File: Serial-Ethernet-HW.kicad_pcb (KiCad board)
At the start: 4 copper layers, 41.1 x 50.7 mm, 52 parts, among them J1 7499111121A, J2 UJ2-MBH-1-SMT-TR, J3 D09P33E4GX00LF, U1 W5500, U2 MPM3612-33, U3 STM32G061GxUx, Y1 ECS-250-10-37B-CTN-TR

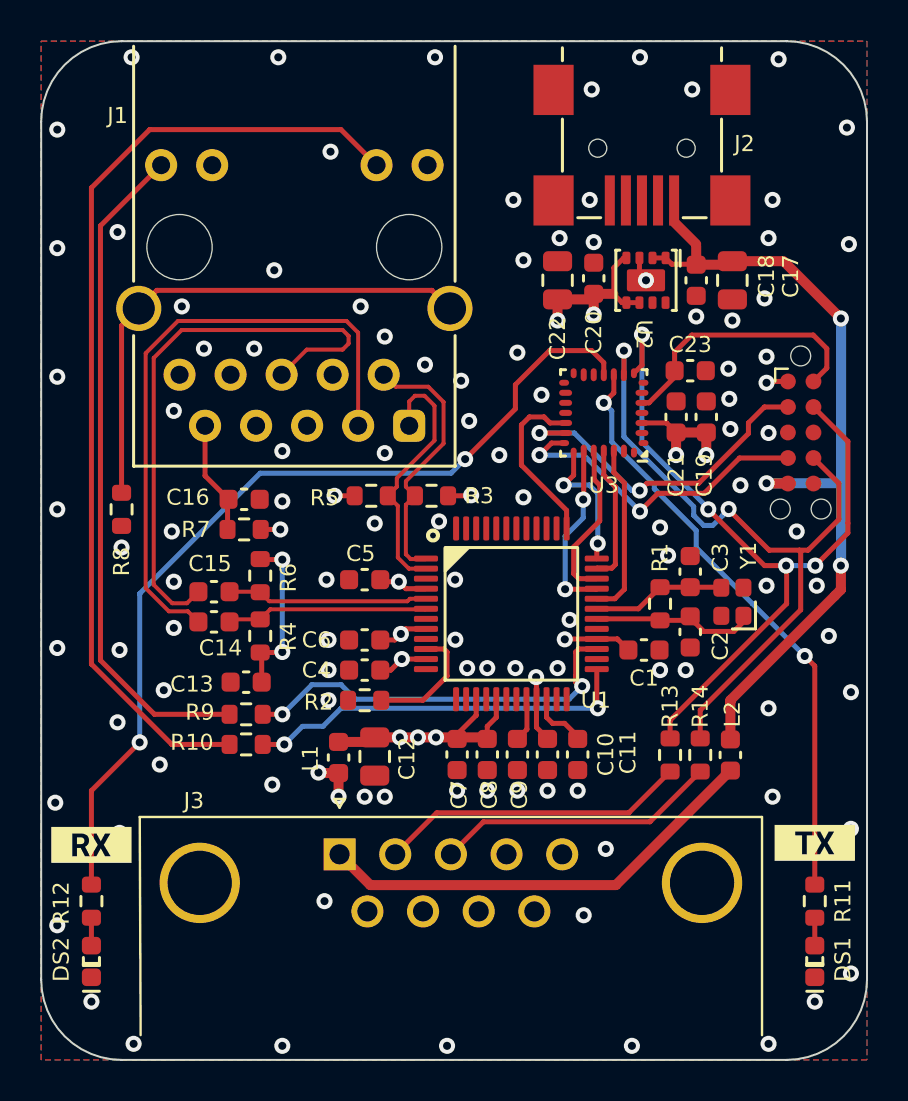
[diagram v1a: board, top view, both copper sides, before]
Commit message: PCB Layout
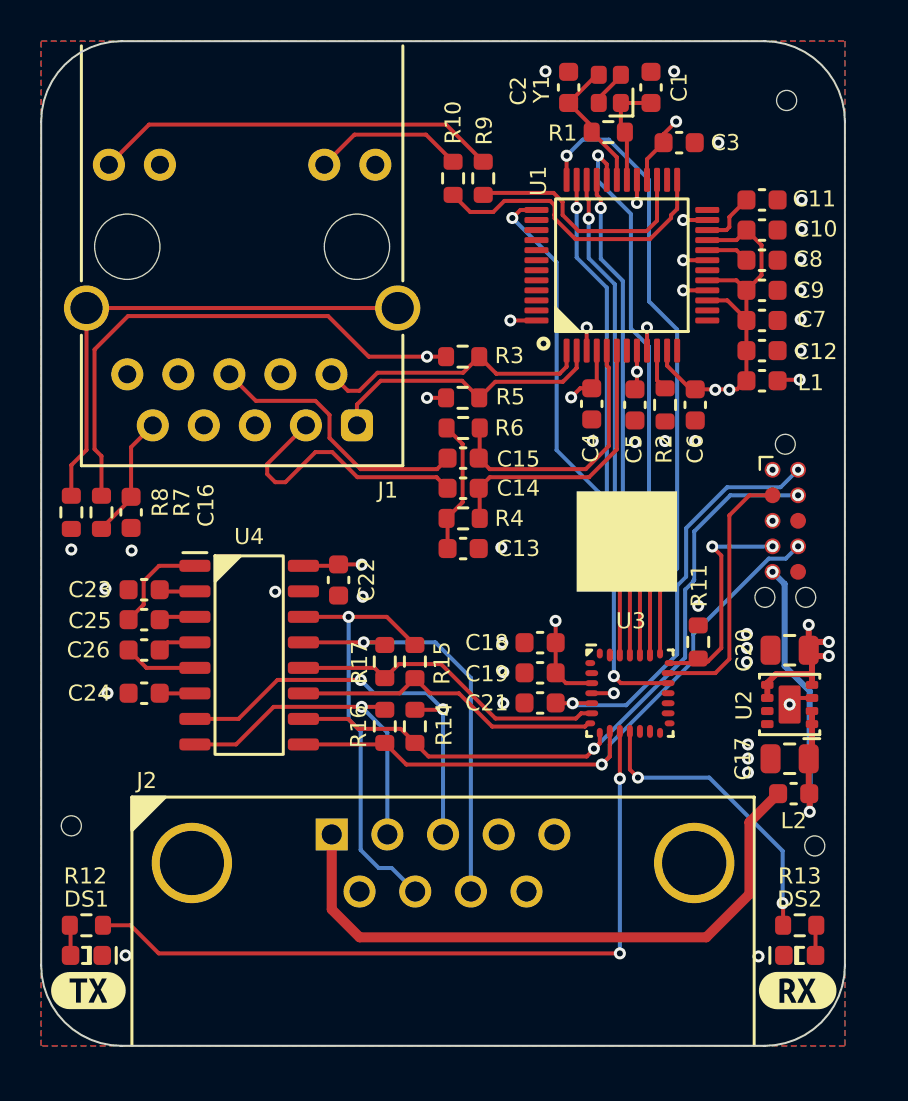
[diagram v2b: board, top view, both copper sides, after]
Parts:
- removed J3: D09P33E4GX00LF, Connector_Dsub:DSUB-9_Male_Horizontal_P2.77x2.84mm_EdgePinOffset7.70mm_Housed_MountingHolesOffset9.12mm
- removed kibuzzard-63E498D1: G***, kibuzzard-63E498D1
- removed kibuzzard-63E498DB: G***, kibuzzard-63E498DB
- added C24: 100n, C_Capacitor:C_0603, F.Cu at (55.1, 82.5)
- added C25: 100n, C_Capacitor:C_0603, F.Cu at (55.1, 78.8)
- added C26: 100n, C_Capacitor:C_0603, F.Cu at (55.1, 80.3)
- added N2: ToolingHole, N_NonPart:ToolingHole_1mm, F.Cu at (87.1, 53.0)
- added N3: ToolingHole, N_NonPart:ToolingHole_1mm, F.Cu at (51.5, 89.0)
- added N4: ToolingHole, N_NonPart:ToolingHole_1mm, F.Cu at (88.5, 90.0)
- added N5: QR 5mm, N_NonPart:QR_5mm_JLC, F.Cu at (79.2, 74.9)
- added R15: 470R, R_Resistor:R_0603, F.Cu at (68.6, 80.9)
- added R16: 470R, R_Resistor:R_0603, F.Cu at (67.1, 84.1)
- added R17: 470R, R_Resistor:R_0603, F.Cu at (67.1, 80.9)
- added U4: ST3232CDR, U_IC:SOIC_16, F.Cu at (60.4, 80.6)
- added kibuzzard-6A8D4FDF: G***, kibuzzard-6A8D4FDF, F.Cu at (52.4, 97.2)
- added kibuzzard-6A8D4FE5: G***, kibuzzard-6A8D4FE5, F.Cu at (87.7, 97.2)
- C1: value 100n -> 18p
- C12: value 10u -> 4u7,10v; footprint C_Capacitor:C_0805 -> C_Capacitor:C_0603
- C17: value 10u -> 22u,10v
- C18, C8: value 100n -> 4u7,10v
- C19, C9: value 4u7 -> 100n
- C20: value 100n -> 22u,10v; footprint C_Capacitor:C_0603 -> C_Capacitor:C_0805
- C22: value 10u -> 100n; footprint C_Capacitor:C_0805 -> C_Capacitor:C_0603
- C3: value 18p -> 100n
- DS1: value LED,YEL -> 150060YS55040
- DS2: value LED,GRN -> 150060VS55040
- J2: value UJ2-MBH-1-SMT-TR -> A-DS_09_A/KG-T4S; footprint J_Connector:USB_Mini_SMD_Horizontal -> J_Connector:DSUB09_Male_Horizontal
- L1, L2: value 600R -> BLM18KG601SN1D
- R10, R12, R13, R14, R9: value 330R -> 470R
- R11: value 330R -> 10K
- moved J2 36.9 mm to (70.0, 90.9), turned to 0 degrees
- moved DS1 36.3 mm to (52.2, 95.5), turned to 180 degrees
- moved DS2 35.3 mm to (87.8, 95.5), turned to 0 degrees
- moved R10 30.0 mm to (70.5, 56.8), turned to -90 degrees
- moved C23 29.3 mm to (55.1, 77.3), turned to 180 degrees
- moved R9 29.2 mm to (72.0, 56.8), turned to 90 degrees
- moved C11 29.1 mm to (85.9, 57.9), turned to 0 degrees
- moved L1 28.2 mm to (85.9, 66.9), turned to 180 degrees
- moved C10 28.2 mm to (85.9, 59.4), turned to 0 degrees
- moved C8 28.1 mm to (85.9, 60.9), turned to 0 degrees
- moved C1 28.0 mm to (80.3, 52.3), turned to -90 degrees
- moved C12 27.9 mm to (85.9, 65.4), turned to 0 degrees
- moved C2 27.8 mm to (76.2, 52.3)
- moved C7 26.4 mm to (85.9, 63.9), turned to 0 degrees
- moved Y1 26.2 mm to (78.3, 52.4)
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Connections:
- C1 pad 1: +3V3 -> GND
- C1 pad 2: GND -> Net-(U1-XI/CLKIN)
- C18 pad 1: +5V -> +3V3
- C2 pad 1: GND -> Net-(U1-XO)
- C2 pad 2: Net-(U1-XI/CLKIN) -> GND
- C21 pad 1: +3V3 -> /Host/NRST
- C23 pad 1: /Host/NRST -> Net-(U4-VS+)
- C3 pad 1: Net-(U1-XO) -> +3V3
- C8 pad 1: +3V3A -> Net-(U1-TOCAP)
- C9 pad 1: Net-(U1-TOCAP) -> +3V3A
- J2 pad 1: +5V -> Net-(J2-Pad1)
- J2 pad 2: unconnected-(J2-D--Pad2) -> /Serial/CN_RXD
- J2 pad 3: unconnected-(J2-D+-Pad3) -> /Serial/CN_TXD
- L2 pad 1: Net-(J3-Pad1) -> Net-(J2-Pad1)
- R11 pad 1: /Host/LED_TX -> /Host/SWCLK
- R11 pad 2: Net-(DS1-A) -> GND
- R12 pad 1: /Host/LED_RX -> /Host/LED_TX
- R12 pad 2: Net-(DS2-A) -> Net-(DS1-A)
- R13 pad 1: Net-(J3-Pad2) -> /Host/LED_RX
- R13 pad 2: /Host/UART_TX -> Net-(DS2-A)
- R14 pad 1: Net-(J3-Pad3) -> /Serial/CN_TXD
- R14 pad 2: /Host/UART_RX -> /Host/UART_TX
- U3 pad 6: unconnected-(U3-PA0-Pad6) -> /Host/CTS
- U3 pad 7: unconnected-(U3-PA1-Pad7) -> /Host/RTS
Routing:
- net Net-(J1-Pad12): track 48.4 -> 7.59 mm
- net Net-(J2-Pad1): track 0.00 -> 31.6 mm
- net /Host/LED_RX: track 45.1 -> 14.9 mm
- net +3V3A: track 26.0 -> 52.6 mm, vias 10 -> 6
- net +5V: track 42.3 -> 18.1 mm, vias 3 -> 2
- net /Ethernet/INT: track 6.97 -> 31.0 mm
- net Net-(J3-Pad1): track 22.4 -> 0.00 mm
- net /Serial/CN_RTS: track 0.00 -> 21.6 mm, vias 0 -> 1
- net /Serial/CN_TXD: track 0.00 -> 21.4 mm, vias 0 -> 2
- net /Ethernet/CS: track 8.66 -> 29.8 mm, vias 0 -> 2
- net /Serial/CN_CTS: track 0.00 -> 20.8 mm, vias 0 -> 1
- net /Ethernet/RST: track 8.57 -> 29.1 mm, vias 0 -> 2
- net /Ethernet/MOSI: track 6.90 -> 24.7 mm, vias 0 -> 2
- net /Ethernet/RXB_P: track 31.1 -> 13.7 mm
- net /Serial/CN_RXD: track 0.00 -> 17.3 mm, vias 0 -> 1
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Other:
- board size 41.1 x 50.7 mm -> 40 x 50 mm
- board text added: "Serial to Ethernet v1.1 Aug 26"
- board text removed: "Serial to Ethernet v1.0b Sep 25"
